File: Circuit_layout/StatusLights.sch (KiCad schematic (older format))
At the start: 33 parts, among them Q1 ZVP4525G, U1 PDM2-S24-S12, U11 TLP293, U12 TLP293, U16 LTC3638

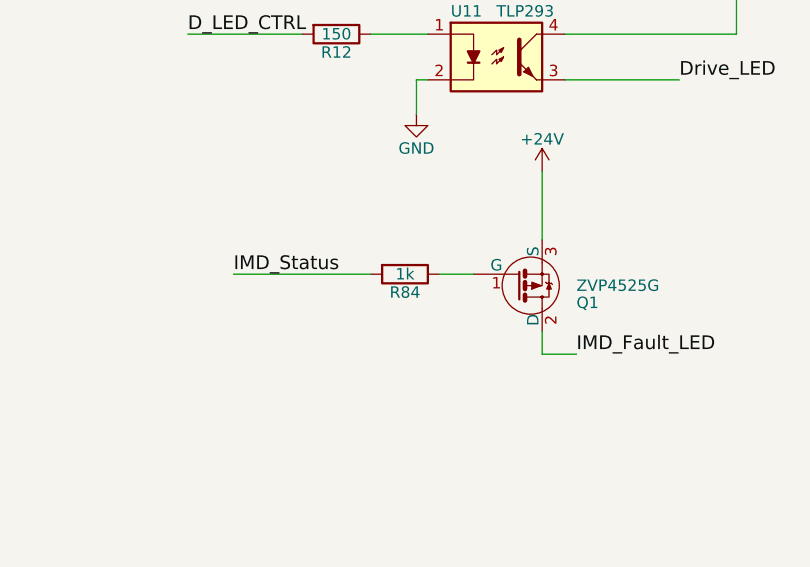
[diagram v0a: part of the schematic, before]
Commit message: small changes
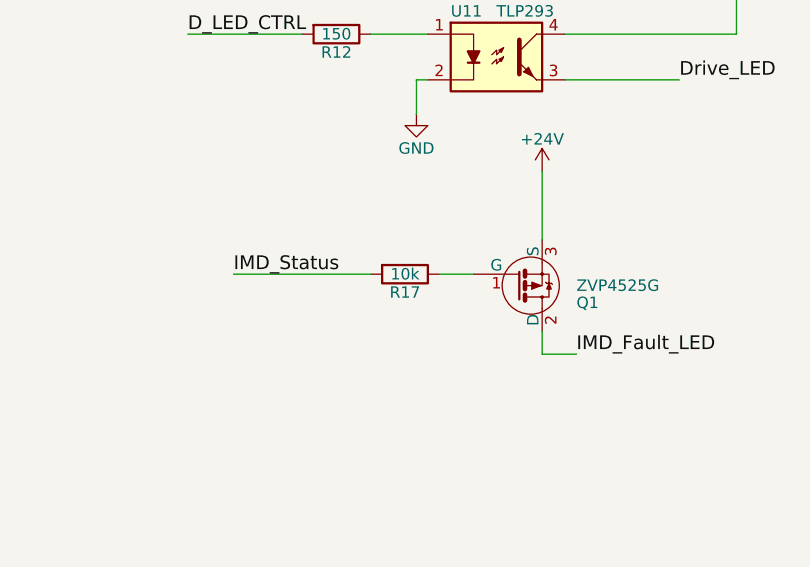
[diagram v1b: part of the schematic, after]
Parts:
- removed R84: 1k, Resistors_SMD:R_0805_HandSoldering, symbol R
- added R17: 10k, Resistors_SMD:R_0805_HandSoldering, symbol R
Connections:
- net IMD_Status: now also R17.2
- net at Q1.1 (G): now also R17.1
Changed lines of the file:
@@
 $EndComp
 $Comp
-L GND #PWR037
+L GND #PWR036
 U 1 1 58AF33D9
 P 4250 1300
-F 0 "#PWR037" H 4250 1050 50  0001 C CNN
+F 0 "#PWR036" H 4250 1050 50  0001 C CNN
 F 1 "GND" H 4250 1150 50  0000 C CNN
 F 2 "" H 4250 1300 50  0000 C CNN
@@
 $EndComp
 $Comp
-L +24V #PWR038
+L +24V #PWR037
 U 1 1 58AF3526
 P 5650 850
-F 0 "#PWR038" H 5650 700 50  0001 C CNN
+F 0 "#PWR037" H 5650 700 50  0001 C CNN
 F 1 "+24V" H 5650 990 50  0000 C CNN
 F 2 "" H 5650 850 50  0000 C CNN
@@
 $EndComp
 $Comp
-L GND #PWR039
+L GND #PWR038
 U 1 1 58AF4273
 P 4250 2500
-F 0 "#PWR039" H 4250 2250 50  0001 C CNN
+F 0 "#PWR038" H 4250 2250 50  0001 C CNN
 F 1 "GND" H 4250 2350 50  0000 C CNN
 F 2 "" H 4250 2500 50  0000 C CNN
@@
 $EndComp
 $Comp
-L +24V #PWR040
+L +24V #PWR039
 U 1 1 58AF427B
 P 5650 2000
-F 0 "#PWR040" H 5650 1850 50  0001 C CNN
+F 0 "#PWR039" H 5650 1850 50  0001 C CNN
 F 1 "+24V" H 5650 2140 50  0000 C CNN
 F 2 "" H 5650 2000 50  0000 C CNN
@@
 $EndComp
 $Comp
-L GND #PWR041
+L GND #PWR040
 U 1 1 58B26825
 P 8750 1200
-F 0 "#PWR041" H 8750 950 50  0001 C CNN
+F 0 "#PWR040" H 8750 950 50  0001 C CNN
 F 1 "GND" H 8750 1050 50  0000 C CNN
 F 2 "" H 8750 1200 50  0000 C CNN
@@
 $EndComp
 $Comp
-L GND #PWR042
+L GND #PWR041
 U 1 1 58B26F4E
 P 8750 1650
-F 0 "#PWR042" H 8750 1400 50  0001 C CNN
+F 0 "#PWR041" H 8750 1400 50  0001 C CNN
 F 1 "GND" H 8750 1500 50  0000 C CNN
 F 2 "" H 8750 1650 50  0000 C CNN
@@
 $EndComp
 $Comp
-L GND #PWR043
+L GND #PWR042
 U 1 1 58B272AA
 P 8750 2100
-F 0 "#PWR043" H 8750 1850 50  0001 C CNN
+F 0 "#PWR042" H 8750 1850 50  0001 C CNN
 F 1 "GND" H 8750 1950 50  0000 C CNN
 F 2 "" H 8750 2100 50  0000 C CNN
@@
 $EndComp
 $Comp
-L GND #PWR044
+L GND #PWR043
 U 1 1 58B27330
 P 8750 2550
-F 0 "#PWR044" H 8750 2300 50  0001 C CNN
+F 0 "#PWR043" H 8750 2300 50  0001 C CNN
 F 1 "GND" H 8750 2400 50  0000 C CNN
 F 2 "" H 8750 2550 50  0000 C CNN
@@
 Blue
 $Comp
-L +5V #PWR045
+L +5V #PWR044
 U 1 1 58B2809B
 P 10250 1100
-F 0 "#PWR045" H 10250 950 50  0001 C CNN
+F 0 "#PWR044" H 10250 950 50  0001 C CNN
 F 1 "+5V" H 10250 1240 50  0000 C CNN
 F 2 "" H 10250 1100 50  0000 C CNN
@@
 Text HLabel 1250 2200 0    60   Input ~ 0
 Spare_Blue
-$Comp
-L R R84
-U 1 1 58BBA9F7
-P 4200 3200
-F 0 "R84" V 4280 3200 50  0000 C CNN
-F 1 "1k" V 4200 3200 50  0000 C CNN
-F 2 "Resistors_SMD:R_0805_HandSoldering" V 4130 3200 50  0001 C CNN
-F 3 "" H 4200 3200 50  0000 C CNN
-F 4 "P1.00KCCT-ND" V 4200 3200 60  0001 C CNN "DigiKey P/N"
-F 5 "http://www.digikey.com/product-detail/en/panasonic-electronic-components/ERJ-6ENF1001V/P1.00KCCT-ND/118957" V 4200 3200 60  0001 C CNN "URL"
-F 6 "ERJ-6ENF1001V" V 4200 3200 60  0001 C CNN "Man P/N"
-	1    4200 3200
-	0    1    1    0
-$EndComp
 Text GLabel 1250 650  0    60   Input ~ 0
 RTDS
@@
 	4800 3550 4950 3550
 $Comp
-L +24V #PWR046
+L +24V #PWR045
 U 1 1 58C523A5
 P 4800 2750
-F 0 "#PWR046" H 4800 2600 50  0001 C CNN
+F 0 "#PWR045" H 4800 2600 50  0001 C CNN
 F 1 "+24V" H 4800 2890 50  0000 C CNN
 F 2 "" H 4800 2750 50  0000 C CNN
@@
 HV-
 $Comp
-L PWR_FLAG #FLG047
+L PWR_FLAG #FLG046
 U 1 1 58C1AF3D
 P 3600 5200
-F 0 "#FLG047" H 3600 5295 50  0001 C CNN
+F 0 "#FLG046" H 3600 5295 50  0001 C CNN
 F 1 "PWR_FLAG" H 3600 5380 50  0000 C CNN
 F 2 "" H 3600 5200 50  0000 C CNN
@@
 NoConn ~ 8650 5700
 $Comp
-L GND #PWR048
+L GND #PWR047
 U 1 1 58D3C796
 P 9400 5950
-F 0 "#PWR048" H 9400 5700 50  0001 C CNN
+F 0 "#PWR047" H 9400 5700 50  0001 C CNN
 F 1 "GND" H 9400 5800 50  0000 C CNN
 F 2 "" H 9400 5950 50  0000 C CNN
@@
 Text Notes 2450 -100 0    60   ~ 0
 U11/12: Verify that these will supply necessary current. Add high side switch on output if necessary. Also could be accomplished with NMOS followed by PMOS
+$Comp
+L R R17
+U 1 1 58D617C3
+P 4200 3200
+F 0 "R17" V 4280 3200 50  0000 C CNN
+F 1 "10k" V 4200 3200 50  0000 C CNN
+F 2 "Resistors_SMD:R_0805_HandSoldering" V 4130 3200 50  0001 C CNN
+F 3 "" H 4200 3200 50  0000 C CNN
+F 4 "P10.0KCCT-ND" V 4200 3200 60  0001 C CNN "DigiKey P/N"
+F 5 "http://www.digikey.com/product-detail/en/panasonic-electronic-components/ERJ-6ENF1002V/P10.0KCCT-ND/119248" V 4200 3200 60  0001 C CNN "URL"
+F 6 "ERJ-6ENF1002V" V 4200 3200 60  0001 C CNN "Man P/N"
+	1    4200 3200
+	0    1    1    0
+$EndComp
 $EndSCHEMATC
